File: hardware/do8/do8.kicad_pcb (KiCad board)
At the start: 2 copper layers, 62.4 x 51 mm, 46 parts, among them J3 PHOENIX_MKDSO_2.5_3_L, J4 PHOENIX_MKDSO_2.5_3_L, J5 PHOENIX_MKDSO_2.5_3_R, J6 PHOENIX_MKDSO_2.5_3_R, Q1 BSP75N, Q2 BSP75N, Q3 BSP75N, Q4 BSP75N, Q5 BSP75N, Q6 BSP75N, Q7 BSP75N, Q8 BSP75N, U1 PHOENIX-BC178, U2 ATmega32U4-A, U3 MCP2551-I-SN, U5 LM78L05_SO8, Y1 3M6834

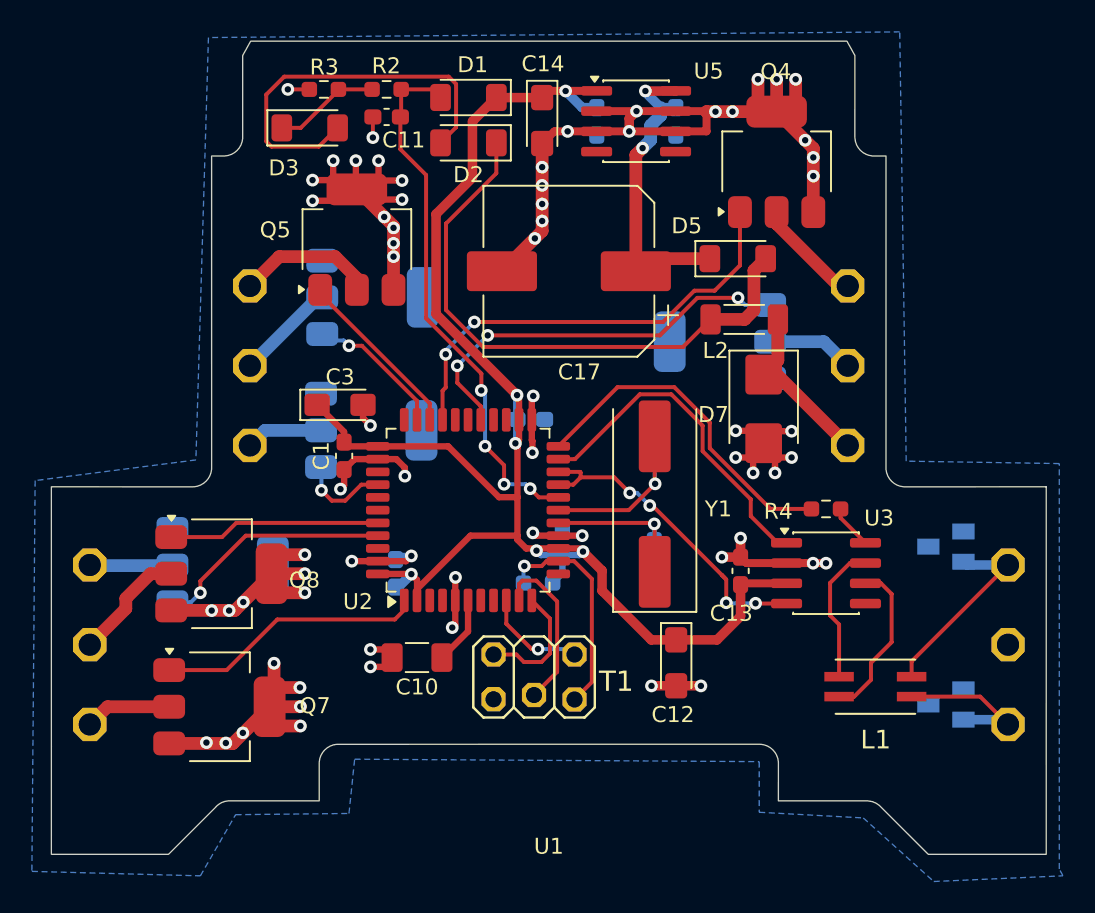
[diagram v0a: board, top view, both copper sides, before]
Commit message: Ordered PCB
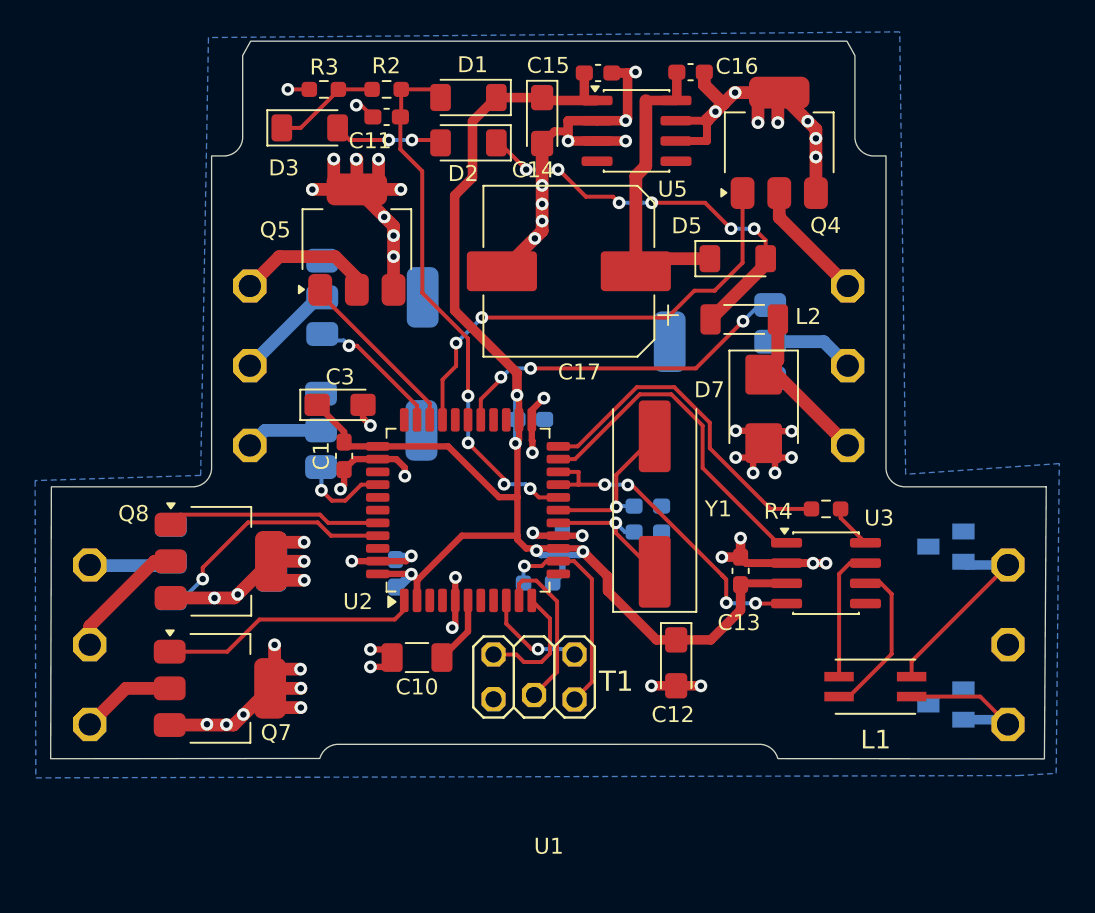
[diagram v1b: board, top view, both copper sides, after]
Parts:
- C15, C16: moved to F.Cu
- U1: footprint mylib:phoenix-bc178-reduced-1 -> mylib:phoenix-bc178-reduced-3
- moved C4 3.73 mm to (154.3, 97.5), turned to 180 degrees
- moved C16 3.22 mm to (157.0, 70.3), turned to 0 degrees
- moved C15 3.04 mm to (151.2, 70.4), turned to 0 degrees
- moved C5 1.46 mm to (154.3, 99.2), turned to 180 degrees
- moved Q4 1.21 mm to (162.5, 74.8)
- moved Q7 1.15 mm to (127.4, 109.0)
- moved Q8 0.78 mm to (127.5, 101.0)
- moved U5 0.60 mm to (153.6, 74.0)
- moved Q1 0.27 mm to (127.5, 101.0)
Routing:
- net Net-(D2-A): track 24.7 -> 6.85 mm, vias 0 -> 2
- net Net-(D2-K): track 36.6 -> 25.8 mm, vias 0 -> 6
- net GNDD: track 166.5 -> 161.8 mm, vias 67 -> 62
- net Net-(Q6-IN): track 25.6 -> 22.0 mm
- net Net-(D5-K): track 20.2 -> 18.5 mm, vias 2 -> 0
- net VCC: track 100.2 -> 98.9 mm, vias 6 -> 5
- net Net-(Q4-IN): track 28.4 -> 29.6 mm
- net Net-(U2-XTAL2): track 10.1 -> 9.07 mm
- net Net-(U2-XTAL1): track 11.2 -> 10.3 mm
- net /DO0: track 6.81 -> 7.61 mm
- net Net-(Q1-IN): track 15.0 -> 15.7 mm
- net /DO4: track 7.33 -> 7.92 mm
- net Net-(Q7-IN): track 16.9 -> 16.4 mm
- net /DO3: track 5.44 -> 5.95 mm
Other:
- board size 62.4 x 51 mm -> 62.4 x 45 mm
